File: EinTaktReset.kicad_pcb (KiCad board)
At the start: 2 copper layers, 100 x 160 mm, 59 parts, among them IC1 74LS624, J1 3PinTerminalBlocktg, J2 3PinTerminalBlocktg, J3 2PinTerminalBlocktg, J4 3PinTerminalBlocktg, J5 2PinTerminalBlocktg, P1 CONN_02X10, P4 CONN_02X10, SW1 SWITCH_INV, SW10 SPST, SW11 SPST, SW12 SPST, SW13 SPST, SW2 SWITCH_INV, SW3 SPST, SW4 SPST, SW5 SPST, SW6 SWITCH_INV, SW7 SPST, SW8 SPST, SW9 SPST, U1 74LS132, U2 74540En, U3 74HCT541_PWR, U4 74LS32, U5 74LS00

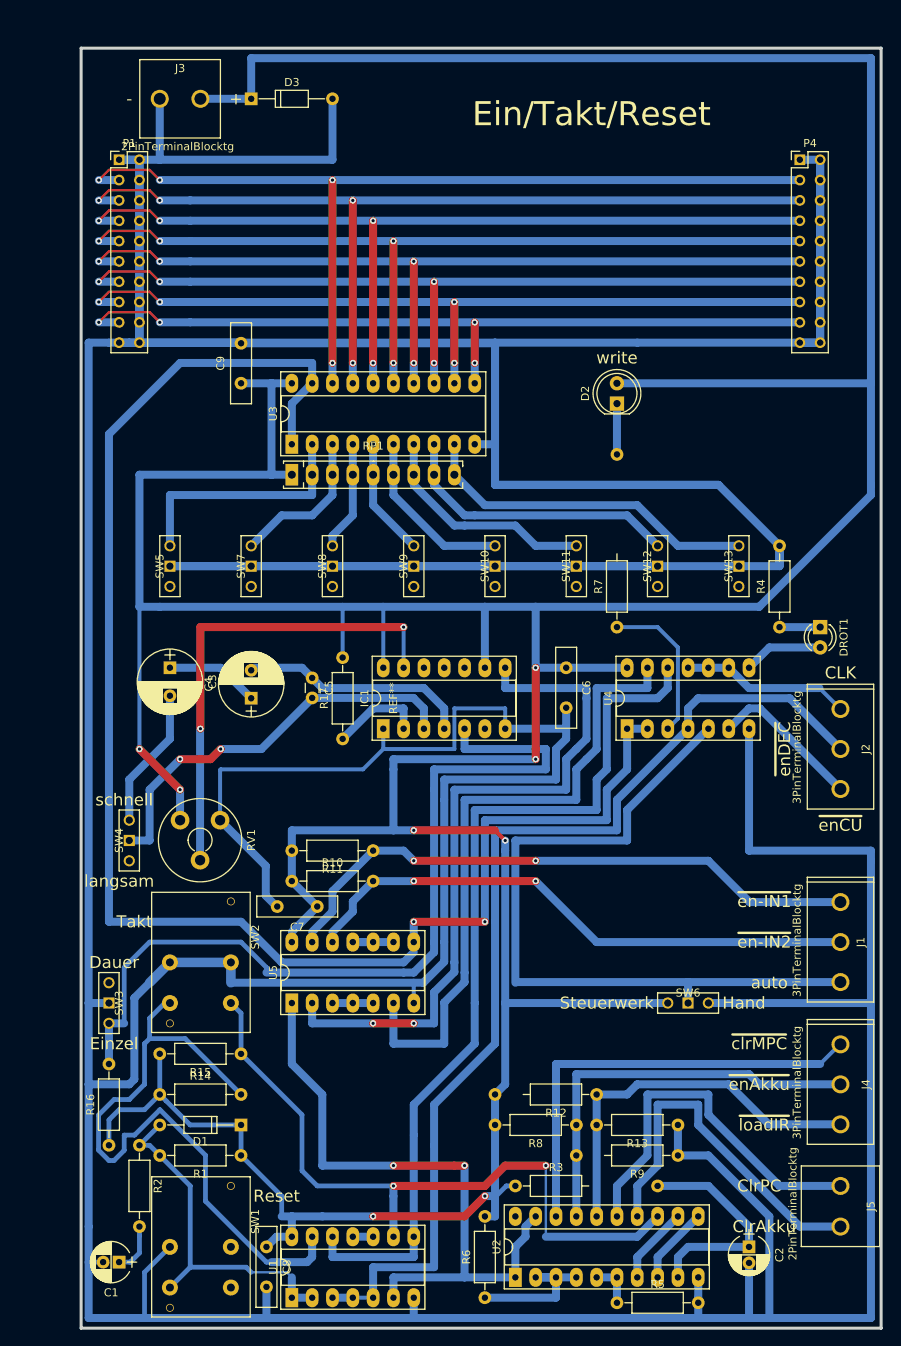
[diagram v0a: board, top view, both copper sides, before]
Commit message: EinTaktReset
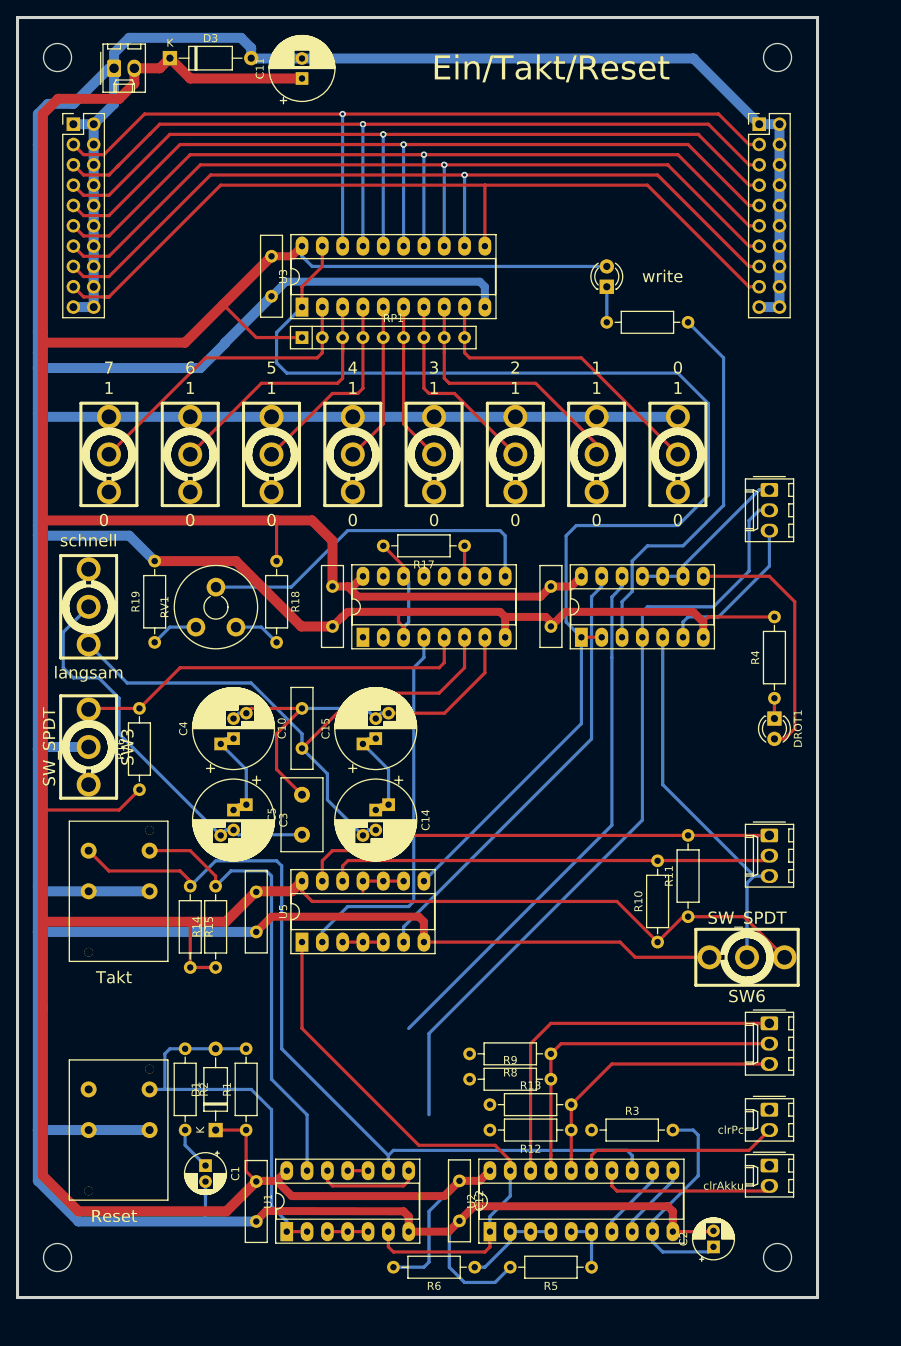
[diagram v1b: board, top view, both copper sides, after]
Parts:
- removed IC1: 74LS624, Housings_DIP:DIP-14_W7.62mm_Socket_LongPads
- removed the REF** at (146.1, 186.7)
- added C10: C, Capacitor_THT:C_Disc_D10.0mm_W2.5mm_P5.00mm, F.Cu at (73.7, 114.2)
- added C11: CP, Capacitor_THT:CP_Radial_D8.0mm_P2.50mm, F.Cu at (73.7, 30.5)
- added C12: 100n, Capacitor_THT:C_Disc_D10.0mm_W2.5mm_P5.00mm, F.Cu at (93.3, 168.3)
- added C13: 100n, Capacitor_THT:C_Disc_D10.0mm_W2.5mm_P5.00mm, F.Cu at (77.5, 94.0)
- added C14: CP, Capacitor_THT:CP_Radial_D10.0mm_P2.50mm_P5.00mm, F.Cu at (82.9, 121.9)
- added C15: CP, Capacitor_THT:CP_Radial_D10.0mm_P2.50mm_P5.00mm, F.Cu at (82.9, 113.0)
- added J6: Conn_01x02, Connector_Molex:Molex_KK-254_AE-6410-02A_1x02_P2.54mm_Vertical, F.Cu at (132.1, 166.4)
- added R18: 10k, Resistor_THT:R_Axial_DIN0207_L6.3mm_D2.5mm_P10.16mm_Horizontal, F.Cu at (70.5, 90.8)
- added R19: 10k, Resistor_THT:R_Axial_DIN0207_L6.3mm_D2.5mm_P10.16mm_Horizontal, F.Cu at (55.2, 101.0)
- added REF**: EuroBoard160mmX100mm_holes_keepout, bonsai:EuroBoard160mmX100mm_holes_keepout, F.Cu at (38.1, 22.9)
- added U6: 74HC4046, Package_DIP:DIP-16_W7.62mm_Socket_LongPads, F.Cu at (81.3, 100.3)
- C1, C2: footprint Capacitors_ThroughHole:CP_Radial_D5.0mm_P2.00mm -> Capacitor_THT:CP_Radial_D5.0mm_P2.00mm
- C3: value 220 µ -> CP; footprint Capacitors_ThroughHole:CP_Radial_D8.0mm_P3.50mm -> Capacitor_THT:CP_Radial_D10.0mm_P2.50mm_P5.00mm
- C4: value 220µ -> CP; footprint Capacitors_ThroughHole:CP_Radial_D8.0mm_P3.50mm -> Capacitor_THT:CP_Radial_D10.0mm_P2.50mm_P5.00mm
- C5: value 10n -> C; footprint Capacitors_ThroughHole:C_Disc_D3.0mm_W1.6mm_P2.50mm -> Capacitor_THT:C_Disc_D9.0mm_W5.0mm_P5.00mm
- C6, C7, C8, C9: footprint Capacitors_ThroughHole:C_Disc_D10.0mm_W2.5mm_P5.00mm -> Capacitor_THT:C_Disc_D10.0mm_W2.5mm_P5.00mm
- D1, D3: footprint Diodes_ThroughHole:D_DO-35_SOD27_P10.16mm_Horizontal -> Diode_THT:D_A-405_P10.16mm_Horizontal
- D2: footprint LEDs:LED_D5.0mm -> LED_THT:LED_D3.0mm
- DROT1: footprint LEDs:LED_D3.0mm -> LED_THT:LED_D3.0mm
- J1: value 3PinTerminalBlocktg -> Conn_01x02; footprint 3PinTerminalBlocktg -> Connector_Molex:Molex_KK-254_AE-6410-02A_1x02_P2.54mm_Vertical
- J2, J4: value 3PinTerminalBlocktg -> Conn_01x03; footprint 3PinTerminalBlocktg -> Connector_Molex:Molex_KK-254_AE-6410-03A_1x03_P2.54mm_Vertical
- J3: value 2PinTerminalBlocktg -> Conn_01x03; footprint 2PinTerminalBlocktg -> Connector_Molex:Molex_KK-254_AE-6410-03A_1x03_P2.54mm_Vertical
- J5: value 2PinTerminalBlocktg -> Conn_01x02; footprint 2PinTerminalBlocktg -> Connector_Molex:Molex_KK-254_AE-6410-02A_1x02_P2.54mm_Vertical
- P1, P4: footprint tg_foodprint:Pin_Header_Straight_2x10_Pitch2.00mmBonsai.pretty -> Connector_PinHeader_2.54mm:PinHeader_2x10_P2.54mm_Vertical
- R1, R10, R11, R13, R16, R17, R2, R4, R5, R6, R8: footprint Resistors_ThroughHole:R_Axial_DIN0207_L6.3mm_D2.5mm_P10.16mm_Horizontal -> Resistor_THT:R_Axial_DIN0207_L6.3mm_D2.5mm_P10.16mm_Horizontal
- R12, R9: footprint tg_foodprint:R_Axial_DIN0207_L6.3mm_D2.5mm_P12.7mm_Horizontaltg -> Resistor_THT:R_Axial_DIN0207_L6.3mm_D2.5mm_P10.16mm_Horizontal
- R14, R15: footprint tg_bonsai_proj_spec_libs:R_Axial_DIN0207_L6.3mm_D2.5mm_P10.16mm_Horizontal -> Resistor_THT:R_Axial_DIN0207_L6.3mm_D2.5mm_P10.16mm_Horizontal
- R3: footprint tg_foodprint:R_Axial_DIN0207_L6.3mm_D2.5mm_P17.7mm_Horizontaltg -> Resistor_THT:R_Axial_DIN0207_L6.3mm_D2.5mm_P10.16mm_Horizontal
- R7: footprint tg_foodprint:R_Axial_DIN0207_L6.3mm_D2.5mm_P21.59mm_Horizontaltg -> Resistor_THT:R_Axial_DIN0207_L6.3mm_D2.5mm_P10.16mm_Horizontal
- RP1: footprint Housings_SIP:SIP9_Housing_BigPads -> Resistor_THT:R_Array_SIP9
- RV1: value POT -> Poti 10k
- SW1, SW2: value SWITCH_INV -> Digitast; footprint tg_foodprint:SW_PUSH_LCD_E3_SAxxxx_tg_V2 -> bonsai:Switch_Digitast
- SW10, SW11, SW12, SW13, SW5, SW7, SW8, SW9: footprint tg_foodprint:eintakt_tg_SW_CuK_JS202011CQN_DPDT_Straight -> Switches-Walter:switch_100sp5
- SW3, SW4: value SPST -> SW_SPDT; footprint tg_foodprint:eintakt_tg_SW_CuK_JS202011CQN_DPDT_Straight -> Switches-Walter:switch_100sp5
- SW6: value SWITCH_INV -> SW_SPDT; footprint tg_foodprint:eintakt_tg_SW_CuK_JS202011CQN_DPDT_Straight -> Switches-Walter:switch_100sp5
- U1: value 74LS132 -> 74132; footprint Housings_DIP:DIP-14_W7.62mm_Socket_LongPads -> Package_DIP:DIP-14_W7.62mm_Socket_LongPads
- U2: value 74540En -> 74540; footprint Housings_DIP:DIP-20_W7.62mm_Socket_LongPads -> Package_DIP:DIP-20_W7.62mm_Socket_LongPads
- U3: footprint Housings_DIP:DIP-20_W7.62mm_Socket_LongPads -> Package_DIP:DIP-20_W7.62mm_Socket_LongPads
- U4: value 74LS32 -> 7432; footprint Housings_DIP:DIP-14_W7.62mm_Socket_LongPads -> Package_DIP:DIP-14_W7.62mm_Socket_LongPads
- U5: value 74LS00 -> 7400; footprint Housings_DIP:DIP-14_W7.62mm_Socket_LongPads -> Package_DIP:DIP-14_W7.62mm_Socket_LongPads
- moved J1 142.0 mm to (50.2, 29.2), turned to 0 degrees
- moved J3 117.9 mm to (132.1, 125.1), turned to 270 degrees
- moved R10 46.4 mm to (118.1, 138.4), turned to 90 degrees
- moved R16 44.6 mm to (53.3, 119.4)
- moved R11 40.2 mm to (121.9, 135.3), turned to 90 degrees
- moved R7 39.1 mm to (121.9, 61.0), turned to 180 degrees
- moved J2 33.6 mm to (132.1, 81.9)
- moved SW4 32.2 mm to (47.0, 96.5)
- moved SW3 29.6 mm to (47.0, 114.0)
- moved R17 28.5 mm to (94.0, 88.9), turned to 180 degrees
- moved R9 27.7 mm to (94.6, 155.6), turned to 0 degrees
- moved RV1 25.1 mm to (65.4, 99.1), turned to 90 degrees
- moved R13 23.6 mm to (97.2, 158.8), turned to 0 degrees
- moved SW1 23.0 mm to (47.0, 161.9), turned to 90 degrees
- moved R15 21.9 mm to (59.7, 131.4), turned to 270 degrees
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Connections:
- C4 pad 2: Net-(C4-Pad2) -> Net-(C10-Pad2)
- C5 pad 1: Net-(C4-Pad2) -> Net-(C3-Pad2)
- C5 pad 2: Net-(C5-Pad2) -> Net-(C10-Pad2)
- J1 pad 1: en-ln1 -> GND
- J1 pad 2: en-ln2 -> VCC
- J3 pad 1: GND -> en-ln1
- J3 pad 2: VCC -> en-ln2
- J5 pad 1: clrPC -> Net-(J5-Pad1)
- J5 pad 2: clrAkku -> clrPC
- P1 pad 11: GND -> /a4
- P1 pad 13: GND -> /a5
- P1 pad 15: GND -> /a6
- P1 pad 17: GND -> /a7
- P1 pad 2: /a0 -> GND
- P1 pad 3: /a1 -> /a0
- P1 pad 4: /a2 -> GND
- P1 pad 5: /a3 -> /a1
- P1 pad 6: /a4 -> GND
- P1 pad 7: /a5 -> /a2
- P1 pad 8: /a6 -> GND
- P1 pad 9: /a7 -> /a3
- P4 pad 11: GND -> /a4
- P4 pad 13: GND -> /a5
- P4 pad 15: GND -> /a6
- P4 pad 17: GND -> /a7
- P4 pad 2: /a0 -> GND
- P4 pad 3: /a1 -> /a0
- P4 pad 4: /a2 -> GND
- P4 pad 5: /a3 -> /a1
- P4 pad 6: /a4 -> GND
- P4 pad 7: /a5 -> /a2
- P4 pad 8: /a6 -> GND
- P4 pad 9: /a7 -> /a3
- R11 pad 1: en-ln1 -> VCC
- R11 pad 2: VCC -> en-ln1
- R16 pad 2: Net-(IC1-Pad5) -> Net-(R16-Pad2)
- R17 pad 2: VCC -> GND
- RV1 pad 1: VCC -> Net-(R18-Pad2)
- RV1 pad 3: GND -> Net-(R19-Pad1)
- SW1 pad 2: (no net) -> Net-(SW1-Pad2)
- SW3 pad 1: GND -> Net-(R16-Pad2)
- SW3 pad 2: Net-(IC1-Pad5) -> GND
- SW3 pad 3: (no net) -> Net-(SW3-Pad3)
- SW4 pad 1: Net-(C5-Pad2) -> Net-(C10-Pad1)
- SW4 pad 3: (no net) -> Net-(SW4-Pad3)
- SW6 pad 1: auto -> VCC
- SW6 pad 2: GND -> auto
- U2 pad 20: (no net) -> VCC
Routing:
- net GND: track 1113.8 -> 799.3 mm
- net Net-(IC1-Pad5): track 109.1 -> 0.00 mm
- net Net-(C10-Pad1): track 0.00 -> 77.3 mm
- net VCC: track 624.5 -> 557.3 mm, vias 8 -> 0
- net Net-(C10-Pad2): track 0.00 -> 53.6 mm
- net Net-(C5-Pad2): track 51.0 -> 0.00 mm, vias 2 -> 0
- net Net-(R16-Pad2): track 0.00 -> 50.0 mm
- net auto: track 93.4 -> 47.0 mm
- net Net-(U5-Pad2): track 88.5 -> 47.8 mm, vias 2 -> 0
- net Net-(U3-Pad1): track 197.6 -> 159.0 mm, vias 2 -> 0
- net Net-(C3-Pad2): track 17.7 -> 50.6 mm
- net enDEC: track 135.7 -> 103.8 mm
- net Net-(U1-Pad12): track 112.2 -> 80.8 mm
- net Net-(R7-Pad1): track 19.4 -> 49.1 mm
- net Net-(C4-Pad2): track 28.9 -> 0.00 mm
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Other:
- board text added: "0"
- board text added: "1"
- board text added: "2"
- board text added: "3"
- board text added: "4"
- board text added: "5"
- board text added: "6"
- board text added: "7"
- board text added: "clrAkku"
- board text added: "clrPc"
- board text removed: "+"
- board text removed: "-"
- board text removed: "CLK"
- board text removed: "ClrAkku"
- board text removed: "ClrPC"
- board text removed: "Dauer"
- board text removed: "Einzel"
- board text removed: "Hand"
- board text removed: "Steuerwerk"
- board text removed: "auto"
- board text removed: "~clrMPC"
- board text removed: "~en-IN1"
- board text removed: "~en-IN2"
- board text removed: "~enAkku"
- board text removed: "~enCU"
- board text removed: "~enDEC"
- board text removed: "~loadIR"
